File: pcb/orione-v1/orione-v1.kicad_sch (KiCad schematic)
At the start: 15 parts, among them J1 Conn_02x10_Odd_Even, J2 Conn_02x10_Odd_Even, J3 Conn_02x03_Odd_Even

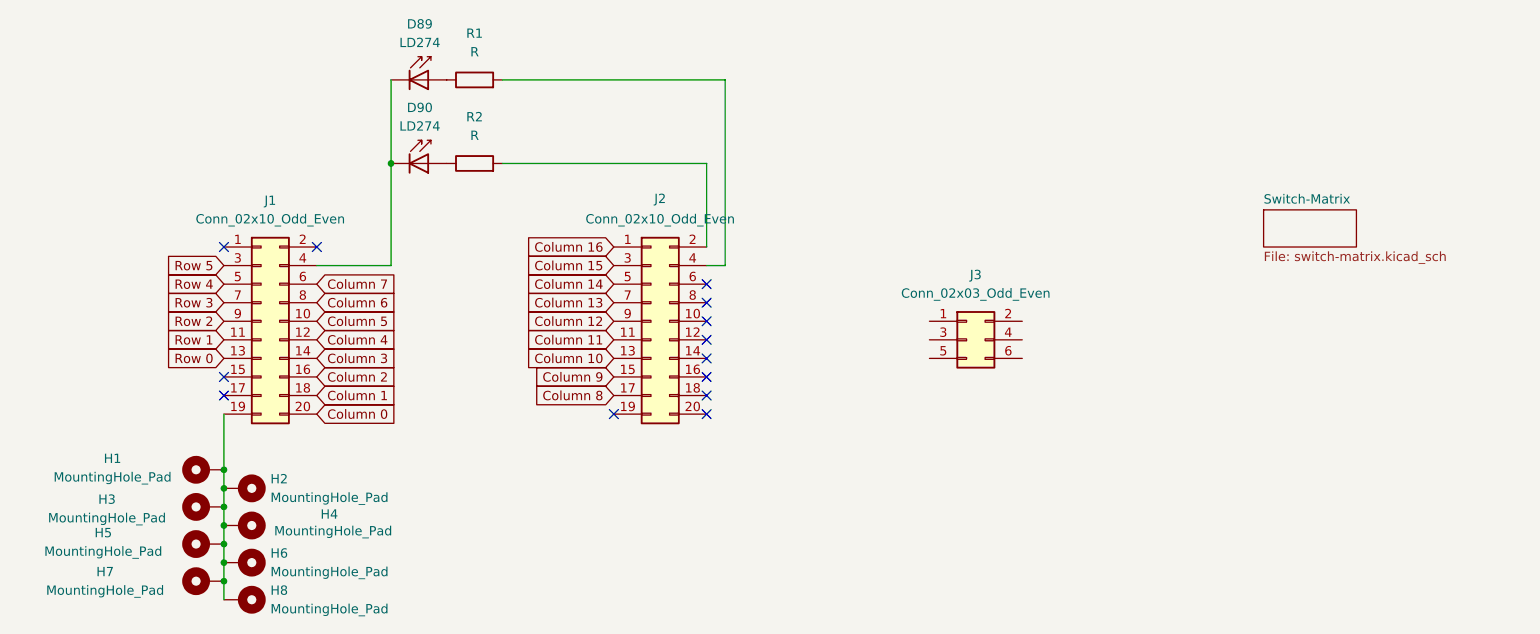
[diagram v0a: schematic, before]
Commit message: pcv v1.1
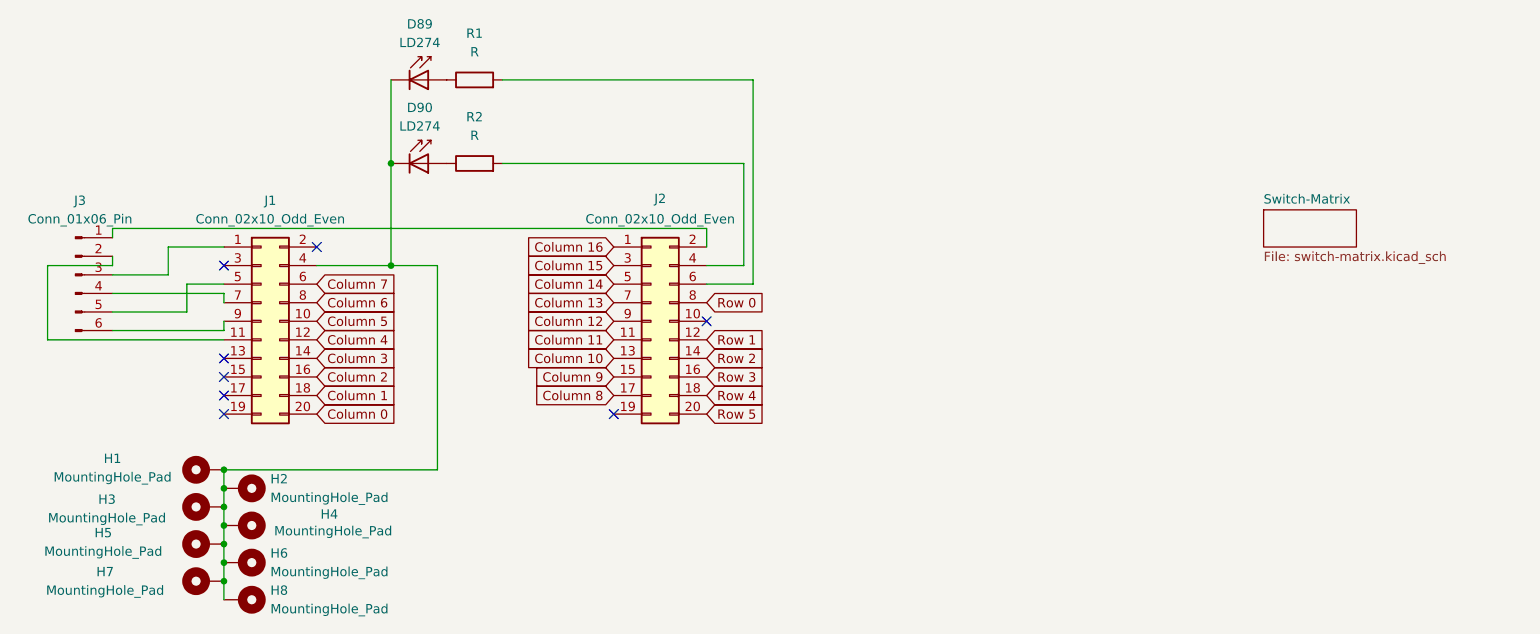
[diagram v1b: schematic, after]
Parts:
- removed J3: Conn_02x03_Odd_Even, Connector_PinHeader_2.54mm:PinHeader_2x03_P2.54mm_Horizontal, symbol Connector_Generic:Conn_02x03_Odd_Even
- added J3: Conn_01x06_Pin, Connector_PinHeader_2.54mm:PinHeader_1x06_P2.54mm_Horizontal, symbol Connector:Conn_01x06_Pin
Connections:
- net Row 0: now also J2.8 (Pin_8); no longer J1.13 (Pin_13)
- net Row 1: now also J2.12 (Pin_12); no longer J1.11 (Pin_11)
- net Row 2: now also J2.14 (Pin_14); no longer J1.9 (Pin_9)
- net Row 3: now also J2.16 (Pin_16); no longer J1.7 (Pin_7)
- net Row 4: now also J2.18 (Pin_18); no longer J1.5 (Pin_5)
- net Row 5: now also J2.20 (Pin_20); no longer J1.3 (Pin_3)
- net at H1.1, H2.1, H3.1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: now also D89.1 (K), D90.1 (K), J1.4 (Pin_4); no longer J1.19 (Pin_19)
- net at J1.1 (Pin_1): now also J3.3 (Pin_3)
- net at R1.2: now also J2.6 (Pin_6); no longer J2.4 (Pin_4)
- net at J2.2 (Pin_2): now also J3.1 (Pin_1); no longer R2.2
- new net: J1.11 (Pin_11), J3.2 (Pin_2)
- new net: J1.5 (Pin_5), J3.5 (Pin_5)
- new net: J1.7 (Pin_7), J3.4 (Pin_4)
- new net: J1.9 (Pin_9), J3.6 (Pin_6)
- new net: J2.4 (Pin_4), R2.2
- no-connect marks 13 -> 8
